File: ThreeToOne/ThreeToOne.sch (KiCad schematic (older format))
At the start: 208 parts, among them SW1 Switch, SW10 Switch, SW100 Switch, SW101 Switch, SW11 Switch, SW12 Switch, SW13 Switch, SW14 Switch, SW15 Switch, SW16 Switch, SW17 REsw, SW18 Switch, SW19 Switch, SW2 Switch, SW20 Switch, SW21 Switch, SW22 Switch, SW23 Switch, SW24 Switch, SW25 Switch, SW26 Switch, SW27 Switch, SW28 Switch, SW29 Switch, SW3 Switch, SW30 Switch, SW31 Switch, SW32 Switch, SW33 Switch, SW34 Switch, SW35 Switch, SW36 Switch, SW37 Switch, SW38 Switch, SW39 Switch, SW4 Switch, SW40 Switch, SW41 Switch, SW42 Switch, SW43 Switch, SW44 Switch, SW45 Switch, SW46 Switch, SW47 Switch, SW48 Switch, SW49 Switch, SW5 Switch, SW50 Switch, SW51 Switch, SW52 Switch, SW53 Switch, SW54 Switch, SW55 Switch, SW56 Switch, SW57 Switch, SW58 Switch, SW59 Switch, SW6 Switch, SW60 Switch, SW61 Switch, SW62 Switch, SW63 Switch, SW64 Switch, SW65 Switch, SW66 Switch, SW67 Switch, SW68 Switch, SW69 Switch, SW7 Switch, SW70 Switch, SW71 Switch, SW72 Switch, SW73 Switch, SW74 Switch, SW75 Switch, SW76 Switch, SW77 Switch, SW78 Switch, SW79 Switch, SW8 Switch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

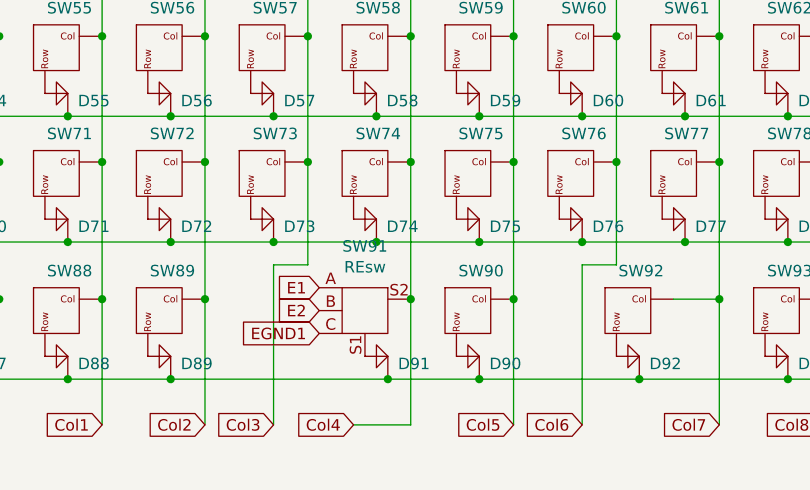
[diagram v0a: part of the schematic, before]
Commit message: Finalization
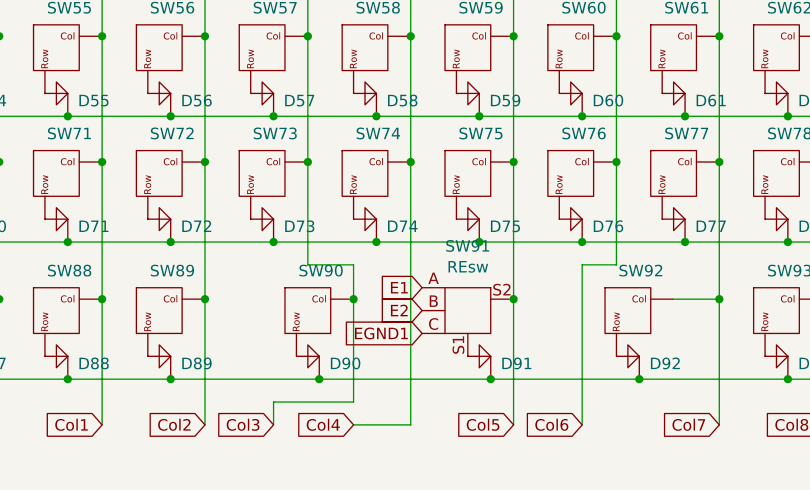
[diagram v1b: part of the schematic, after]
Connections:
- net Col3: now also SW90.1
- net Col4: no longer SW91.S2
- net Col5: now also SW91.S2; no longer SW90.1
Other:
- moved on the sheet: D90, D91, SW90, SW91
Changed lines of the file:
@@
 L KeyboardLibrary:Switch SW90
 U 1 1 60535E84
-P 3200 5500
-F 0 "SW90" H 3158 5773 50  0000 C CNN
-F 1 "Switch" H 3150 5550 50  0001 C CNN
-F 2 "KeyboardFootprints:MX_Choc_Symmetric" H 3200 5500 50  0001 C CNN
-F 3 "" H 3200 5500 50  0001 C CNN
-	1    3200 5500
+P 2500 5500
+F 0 "SW90" H 2458 5773 50  0000 C CNN
+F 1 "Switch" H 2450 5550 50  0001 C CNN
+F 2 "KeyboardFootprints:MX_Choc_Symmetric" H 2500 5500 50  0001 C CNN
+F 3 "" H 2500 5500 50  0001 C CNN
+	1    2500 5500
 	1    0    0    -1
 $EndComp
@@
 L KeyboardLibrary:Diode D90
 U 1 1 60535E7E
-P 3050 5600
-F 0 "D90" H 3194 5567 50  0000 L CNN
-F 1 "Diode" H 3150 5700 50  0001 C CNN
-F 2 "KeyboardFootprints:Diode" H 3150 5700 50  0001 C CNN
-F 3 "" H 3150 5700 50  0001 C CNN
-	1    3050 5600
+P 2350 5600
+F 0 "D90" H 2494 5567 50  0000 L CNN
+F 1 "Diode" H 2450 5700 50  0001 C CNN
+F 2 "KeyboardFootprints:Diode" H 2450 5700 50  0001 C CNN
+F 3 "" H 2450 5700 50  0001 C CNN
+	1    2350 5600
 	1    0    0    -1
 $EndComp
@@
 L KeyboardLibrary:REsw SW91
 U 1 1 60760716
-P 2650 5450
-F 0 "SW91" H 2650 5781 50  0000 C CNN
-F 1 "REsw" H 2650 5690 50  0000 C CNN
-F 2 "KeyboardFootprints:REsw" H 2150 5910 50  0001 C CNN
-F 3 "~" V 2810 5600 50  0001 C CNN
-	1    2650 5450
+P 3100 5450
+F 0 "SW91" H 3100 5781 50  0000 C CNN
+F 1 "REsw" H 3100 5690 50  0000 C CNN
+F 2 "KeyboardFootprints:REsw" H 2600 5910 50  0001 C CNN
+F 3 "~" V 3260 5600 50  0001 C CNN
+	1    3100 5450
 	1    0    0    -1
 $EndComp
@@
 L KeyboardLibrary:Diode D91
 U 1 1 60535EBA
-P 2650 5600
-F 0 "D91" H 2794 5567 50  0000 L CNN
-F 1 "Diode" H 2750 5700 50  0001 C CNN
-F 2 "KeyboardFootprints:Diode" H 2750 5700 50  0001 C CNN
-F 3 "" H 2750 5700 50  0001 C CNN
-	1    2650 5600
+P 3100 5600
+F 0 "D91" H 3244 5567 50  0000 L CNN
+F 1 "Diode" H 3200 5700 50  0001 C CNN
+F 2 "KeyboardFootprints:Diode" H 3200 5700 50  0001 C CNN
+F 3 "" H 3200 5700 50  0001 C CNN
+	1    3100 5600
 	1    0    0    -1
 $EndComp
@@
 Wire Wire Line
 	4650 4750 4650 4200
-Text GLabel 2450 5300 0    50   Input ~ 0
+Text GLabel 2900 5300 0    50   Input ~ 0
 E1
-Text GLabel 2450 5400 0    50   Input ~ 0
+Text GLabel 2900 5400 0    50   Input ~ 0
 E2
-Text GLabel 2450 5500 0    50   Input ~ 0
+Text GLabel 2900 5500 0    50   Input ~ 0
 EGND1
 Connection ~ 7000 3000
@@
 Wire Wire Line
 	2400 4750 2400 5200
-Wire Wire Line
-	2400 5200 2250 5200
 Connection ~ 2400 4750
 Wire Wire Line
@@
 Wire Wire Line
 	4200 5350 4200 5900
-Wire Wire Line
-	2250 5200 2250 5900
 Wire Wire Line
 	1950 5350 1950 5900
@@
 Connection ~ 10200 2000
 Wire Wire Line
+	2850 5900 2600 5900
+Wire Wire Line
+	1800 5700 2450 5700
+Wire Wire Line
+	2850 4750 2850 5900
+Connection ~ 2450 5700
+Wire Wire Line
 	3300 4750 3300 5350
 Wire Wire Line
-	1800 5700 2750 5700
-Connection ~ 2750 5700
-Wire Wire Line
-	2750 5700 3150 5700
-Wire Wire Line
-	2850 5900 2600 5900
-Wire Wire Line
-	2850 4750 2850 5350
-Connection ~ 2850 5350
-Wire Wire Line
-	2850 5350 2850 5900
-Connection ~ 3150 5700
-Wire Wire Line
-	3150 5700 3850 5700
+	2450 5700 3200 5700
+Connection ~ 3200 5700
+Wire Wire Line
+	3200 5700 3850 5700
 Connection ~ 3300 5350
 Wire Wire Line
 	3300 5350 3300 5900
+Wire Wire Line
+	2600 5350 2600 5200
+Wire Wire Line
+	2600 5200 2400 5200
+Wire Wire Line
+	2600 5350 2600 5800
+Wire Wire Line
+	2600 5800 2250 5800
+Wire Wire Line
+	2250 5800 2250 5900
+Connection ~ 2600 5350
 $EndSCHEMATC
